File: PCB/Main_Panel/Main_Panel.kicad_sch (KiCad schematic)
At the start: 3 parts, among them IC1 TCA6424ARGJR, U1 Pico, U2 TLC5947DAP

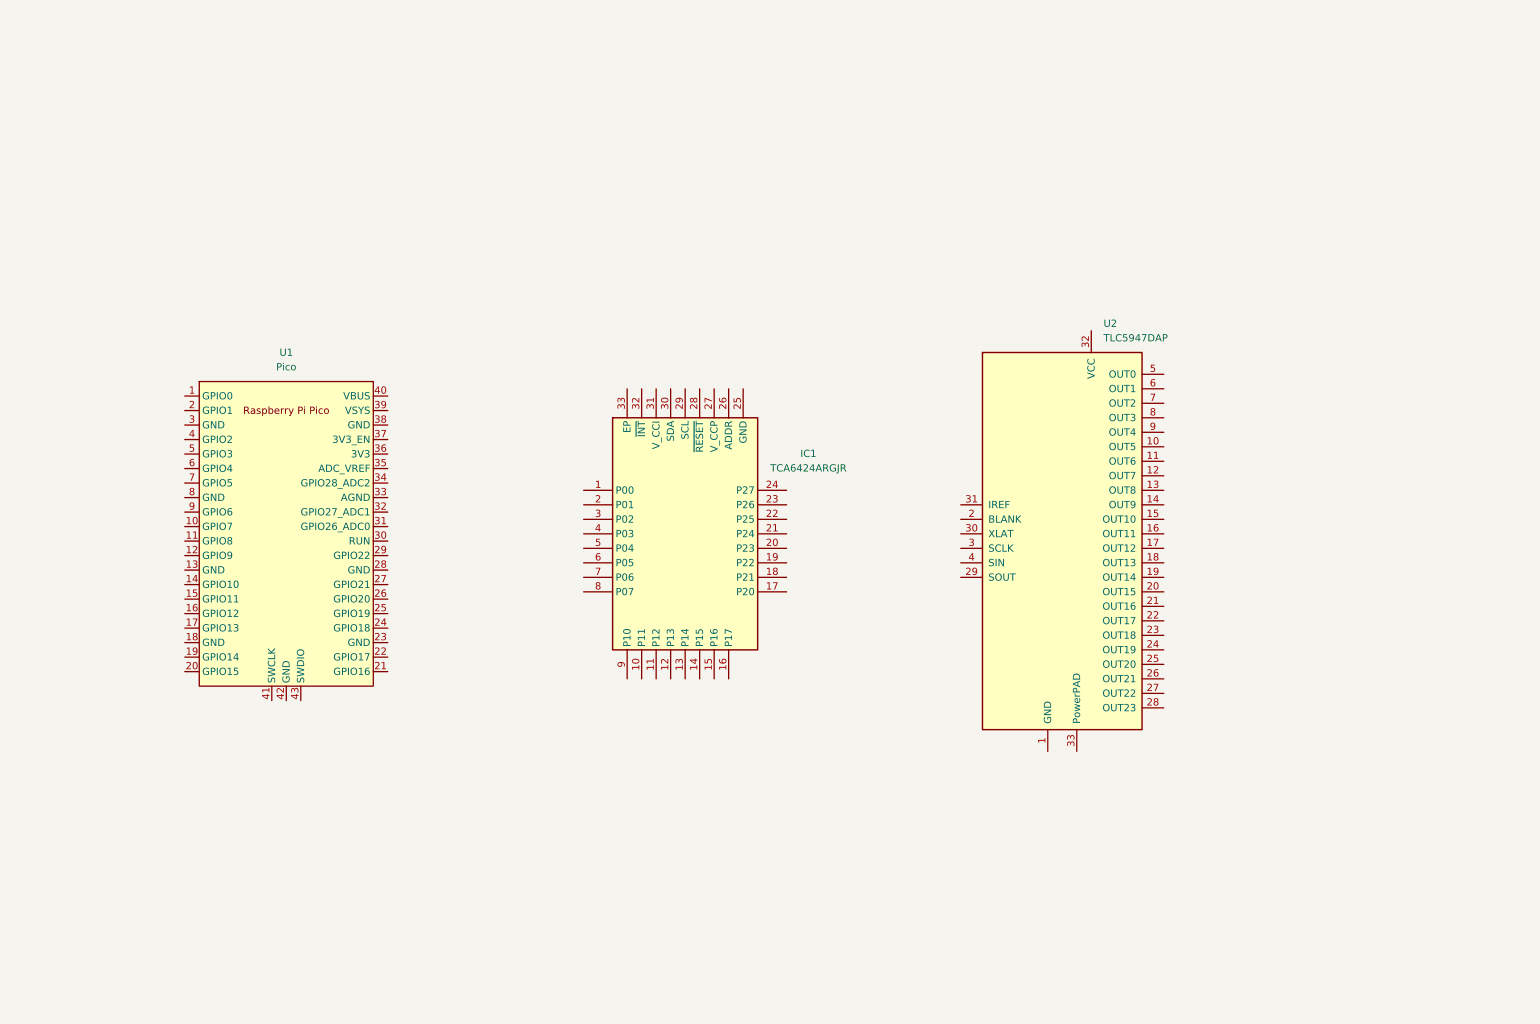
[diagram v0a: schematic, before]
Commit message: PCB Designs
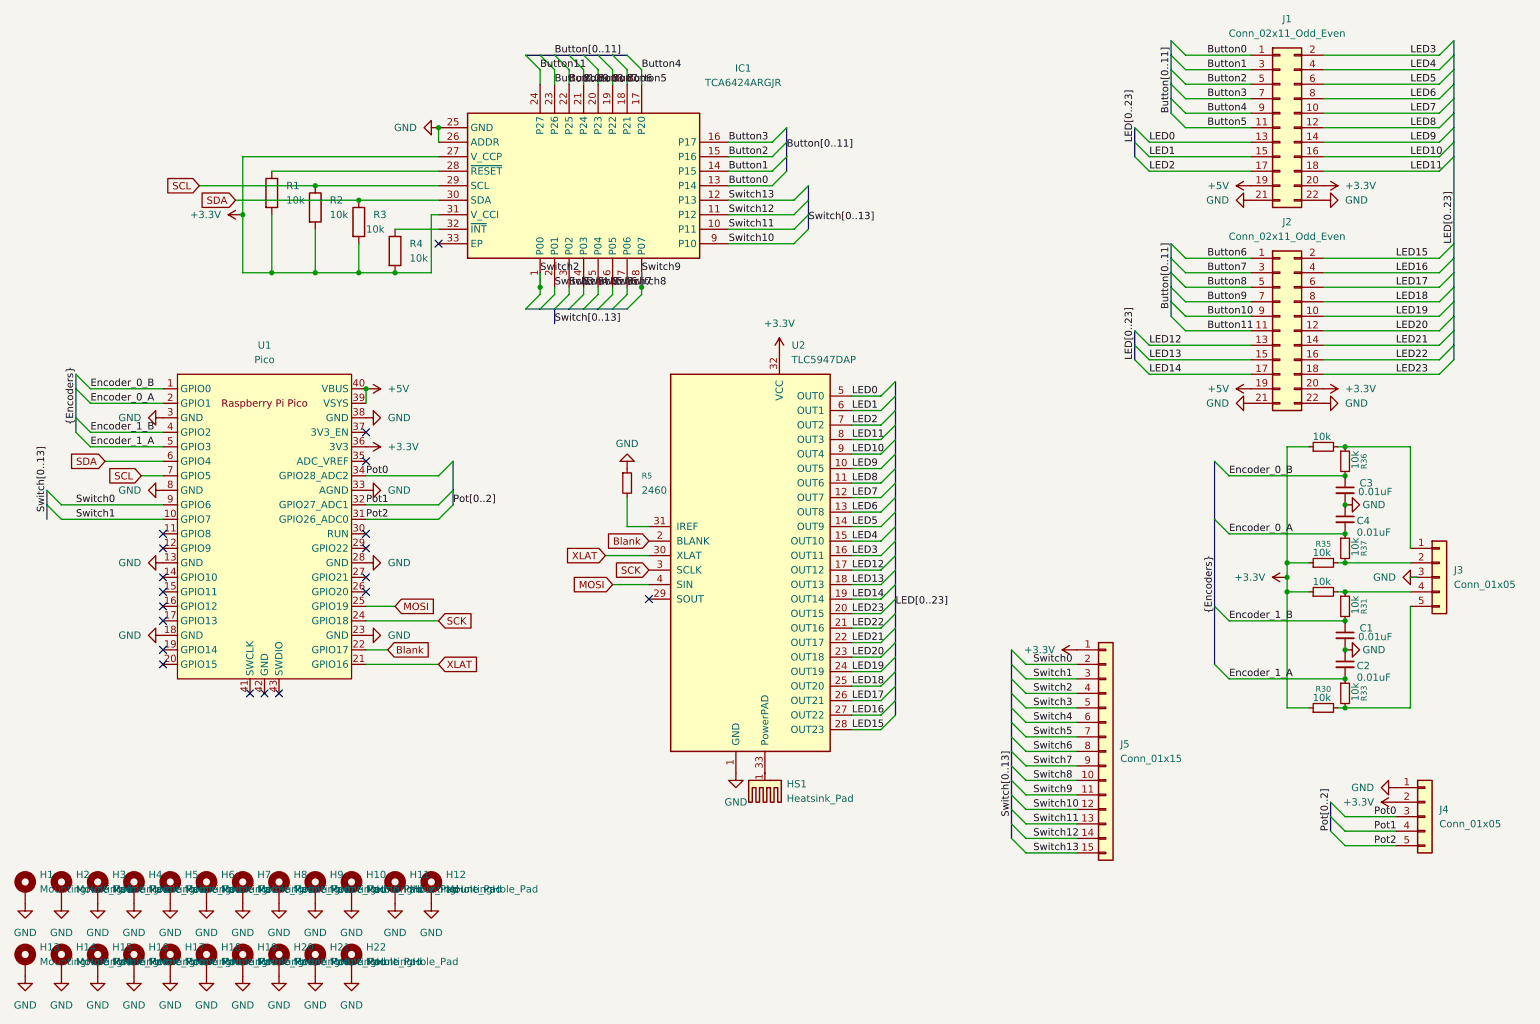
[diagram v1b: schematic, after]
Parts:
- added C1, C2, C3, C4: 0.01uF, Capacitor_SMD:C_0805_2012Metric, symbol Device:C_Small
- added H1, H10, H11, H12, H13, H14, H15, H16, H17, H18, H19, H2, H20, H21, H22, H3, H4, H5, H6, H7, H8, H9: MountingHole_Pad, MountingHole:MountingHole_3.2mm_M3_DIN965_Pad, symbol Mechanical:MountingHole_Pad
- added HS1: Heatsink_Pad, Control_Panel_Footprints:Heat Sink, symbol Mechanical:Heatsink_Pad
- added J1, J2: Conn_02x11_Odd_Even, Connector_PinHeader_2.54mm:PinHeader_2x11_P2.54mm_Vertical, symbol Connector_Generic:Conn_02x11_Odd_Even
- added J3, J4: Conn_01x05, Connector_PinHeader_2.54mm:PinHeader_1x05_P2.54mm_Vertical, symbol Connector_Generic:Conn_01x05
- added J5: Conn_01x15, Connector_PinHeader_2.54mm:PinHeader_1x15_P2.54mm_Vertical, symbol Connector_Generic:Conn_01x15
- added R1, R2, R3, R4: 10k, Resistor_SMD:R_0805_2012Metric, symbol Device:R
- added R30, R31, R32, R33, R34, R35, R36, R37: 10k, Resistor_SMD:R_0805_2012Metric, symbol Device:R_Small
- added R5: 2460, Resistor_SMD:R_0805_2012Metric, symbol Device:R_Small
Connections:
- net Encoder_0_B: now reaches U1.1 (GPIO0)
- net Encoder_0_B: now also C3.1, R36.2
- net Switch1: now reaches U1.10 (GPIO7)
- net Switch1: now also J5.3 (Pin_3)
- net GND: now reaches U1.13 (GND)
- net GND: now also IC1.25 (GND), IC1.26 (ADDR), U1.18 (GND), U1.23 (GND), U1.28 (GND), U1.3 (GND), U1.33 (AGND), U1.38 (GND), U1.8 (GND), U2.1 (GND), C1.2, C2.1, C3.2, C4.1, H1.1, H10.1, H11.1, H12.1, H13.1, H14.1, H15.1, H16.1, H17.1, H18.1, H19.1, H2.1, H20.1, H21.1, H22.1, H3.1, H4.1, H5.1, H6.1, H7.1, H8.1, H9.1, J1.21 (Pin_21), J1.22 (Pin_22), J2.21 (Pin_21), J2.22 (Pin_22), J3.3 (Pin_3), J4.1 (Pin_1), R5.1
- net Encoder_0_A: now reaches U1.2 (GPIO1)
- net Encoder_0_A: now also C4.2, R37.1
- net XLAT: now reaches U1.21 (GPIO16)
- net XLAT: now also U2.30 (XLAT)
- net Blank: now reaches U1.22 (GPIO17)
- net Blank: now also U2.2 (BLANK)
- net SCK: now reaches U1.24 (GPIO18)
- net SCK: now also U2.3 (SCLK)
- net MOSI: now reaches U1.25 (GPIO19)
- net MOSI: now also U2.4 (SIN)
- net Pot2: now reaches U1.31 (GPIO26_ADC0)
- net Pot2: now also J4.5 (Pin_5)
- net Pot1: now reaches U1.32 (GPIO27_ADC1)
- net Pot1: now also J4.4 (Pin_4)
- net Pot0: now reaches U1.34 (GPIO28_ADC2)
- net Pot0: now also J4.3 (Pin_3)
- net +3.3V: now reaches U1.36 (3V3)
- net +3.3V: now also IC1.27 (V_CCP), IC1.31 (V_CCI), U2.32 (VCC), J1.20 (Pin_20), J2.20 (Pin_20), J4.2 (Pin_2), J5.1 (Pin_1), R1.2, R2.2, R3.2, R30.1, R32.1, R34.1, R35.1, R4.2
- net +5V: now reaches U1.39 (VSYS)
- net +5V: now also U1.40 (VBUS), J1.19 (Pin_19), J2.19 (Pin_19)
- net Encoder_1_B: now reaches U1.4 (GPIO2)
- net Encoder_1_B: now also C1.1, R31.2
- net Encoder_1_A: now reaches U1.5 (GPIO3)
- net Encoder_1_A: now also C2.2, R33.1
- net SDA: now reaches U1.6 (GPIO4)
- net SDA: now also IC1.30 (SDA), R3.1
- net SCL: now reaches U1.7 (GPIO5)
- net SCL: now also IC1.29 (SCL), R2.1
- net Switch0: now reaches U1.9 (GPIO6)
- net Switch0: now also J5.2 (Pin_2)
- net Switch2: now reaches IC1.1 (P00)
- net Switch2: now also J5.4 (Pin_4)
- net Switch11: now reaches IC1.10 (P11)
- net Switch11: now also J5.13 (Pin_13)
- net Switch12: now reaches IC1.11 (P12)
- net Switch12: now also J5.14 (Pin_14)
- net Switch13: now reaches IC1.12 (P13)
- net Switch13: now also J5.15 (Pin_15)
- net Button0: now reaches IC1.13 (P14)
- net Button0: now also J1.1 (Pin_1)
- net Button1: now reaches IC1.14 (P15)
- net Button1: now also J1.3 (Pin_3)
- net Button2: now reaches IC1.15 (P16)
- net Button2: now also J1.5 (Pin_5)
- net Button3: now reaches IC1.16 (P17)
- net Button3: now also J1.7 (Pin_7)
- net Button4: now reaches IC1.17 (P20)
- net Button4: now also J1.9 (Pin_9)
- net Button5: now reaches IC1.18 (P21)
- net Button5: now also J1.11 (Pin_11)
- net Button6: now reaches IC1.19 (P22)
- net Button6: now also J2.1 (Pin_1)
- net Switch3: now reaches IC1.2 (P01)
- net Switch3: now also J5.5 (Pin_5)
- net Button7: now reaches IC1.20 (P23)
- net Button7: now also J2.3 (Pin_3)
- net Button8: now reaches IC1.21 (P24)
- net Button8: now also J2.5 (Pin_5)
- net Button9: now reaches IC1.22 (P25)
- net Button9: now also J2.7 (Pin_7)
- net Button10: now reaches IC1.23 (P26)
- net Button10: now also J2.9 (Pin_9)
- net Button11: now reaches IC1.24 (P27)
- net Button11: now also J2.11 (Pin_11)
- net at IC1.28 (~{RESET}): now also R1.1
- net Switch4: now reaches IC1.3 (P02)
- net Switch4: now also J5.6 (Pin_6)
- net at IC1.32 (~{INT}): now also R4.1
- net Switch5: now reaches IC1.4 (P03)
- net Switch5: now also J5.7 (Pin_7)
- net Switch6: now reaches IC1.5 (P04)
- net Switch6: now also J5.8 (Pin_8)
- net Switch7: now reaches IC1.6 (P05)
- net Switch7: now also J5.9 (Pin_9)
- net Switch8: now reaches IC1.7 (P06)
- net Switch8: now also J5.10 (Pin_10)
- net Switch9: now reaches IC1.8 (P07)
- net Switch9: now also J5.11 (Pin_11)
- net Switch10: now reaches IC1.9 (P10)
- net Switch10: now also J5.12 (Pin_12)
- net LED9: now reaches U2.10 (OUT5)
- net LED9: now also J1.14 (Pin_14)
- net LED8: now reaches U2.11 (OUT6)
- net LED8: now also J1.12 (Pin_12)
- net LED7: now reaches U2.12 (OUT7)
- net LED7: now also J1.10 (Pin_10)
- net LED6: now reaches U2.13 (OUT8)
- net LED6: now also J1.8 (Pin_8)
- net LED5: now reaches U2.14 (OUT9)
- net LED5: now also J1.6 (Pin_6)
- net LED4: now reaches U2.15 (OUT10)
- net LED4: now also J1.4 (Pin_4)
- net LED3: now reaches U2.16 (OUT11)
- net LED3: now also J1.2 (Pin_2)
- net LED12: now reaches U2.17 (OUT12)
- net LED12: now also J2.13 (Pin_13)
- net LED13: now reaches U2.18 (OUT13)
- net LED13: now also J2.15 (Pin_15)
- net LED14: now reaches U2.19 (OUT14)
- net LED14: now also J2.17 (Pin_17)
- net LED23: now reaches U2.20 (OUT15)
- net LED23: now also J2.18 (Pin_18)
- net LED22: now reaches U2.21 (OUT16)
- net LED22: now also J2.16 (Pin_16)
- net LED21: now reaches U2.22 (OUT17)
- net LED21: now also J2.14 (Pin_14)
- net LED20: now reaches U2.23 (OUT18)
- net LED20: now also J2.12 (Pin_12)
- net LED19: now reaches U2.24 (OUT19)
- net LED19: now also J2.10 (Pin_10)
- net LED18: now reaches U2.25 (OUT20)
- net LED18: now also J2.8 (Pin_8)
- net LED17: now reaches U2.26 (OUT21)
- net LED17: now also J2.6 (Pin_6)
- net LED16: now reaches U2.27 (OUT22)
- net LED16: now also J2.4 (Pin_4)
- net LED15: now reaches U2.28 (OUT23)
- net LED15: now also J2.2 (Pin_2)
- net at U2.31 (IREF): now also R5.2
- net at U2.33 (PowerPAD): now also HS1.1
- net LED0: now reaches U2.5 (OUT0)
- net LED0: now also J1.13 (Pin_13)
- net LED1: now reaches U2.6 (OUT1)
- net LED1: now also J1.15 (Pin_15)
- net LED2: now reaches U2.7 (OUT2)
- net LED2: now also J1.17 (Pin_17)
- net LED11: now reaches U2.8 (OUT3)
- net LED11: now also J1.18 (Pin_18)
- net LED10: now reaches U2.9 (OUT4)
- net LED10: now also J1.16 (Pin_16)
- new net: J3.4 (Pin_4), R31.1, R32.2
- new net: J3.1 (Pin_1), R34.2, R36.1
- new net: J3.2 (Pin_2), R35.2, R37.2
- new net: J3.5 (Pin_5), R30.2, R33.2
- no-connect marks 0 -> 19
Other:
- moved on the sheet: IC1, U1, U2
